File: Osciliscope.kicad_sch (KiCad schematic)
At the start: 65 parts, among them J1 Conn_01x09_Socket, J2 Conn_01x04_Socket, J3 U.FL, J4 Conn_01x04_Socket, J5 USB_C_Receptacle_USB2.0_14P, J6 Conn_01x02_MountingPin, J7 U.FL, SW1 RotaryEncoder_Switch, SW2 SW_SPST, SW3 SW_Nidec_CAS-120A1, SW4 SW_Nidec_CAS-120A1, SW5 RotaryEncoder_Switch, SW6 RotaryEncoder_Switch, U1 MCP1700x-330xxMB, U2 ADC082S101, U3 IP2721, U4 AZ1084-5.0, U5 TLV9061xDBV, U6 TLV9061xDBV, U7 TLV9061xDBV, U8 MCP4251-104E/ML-ND

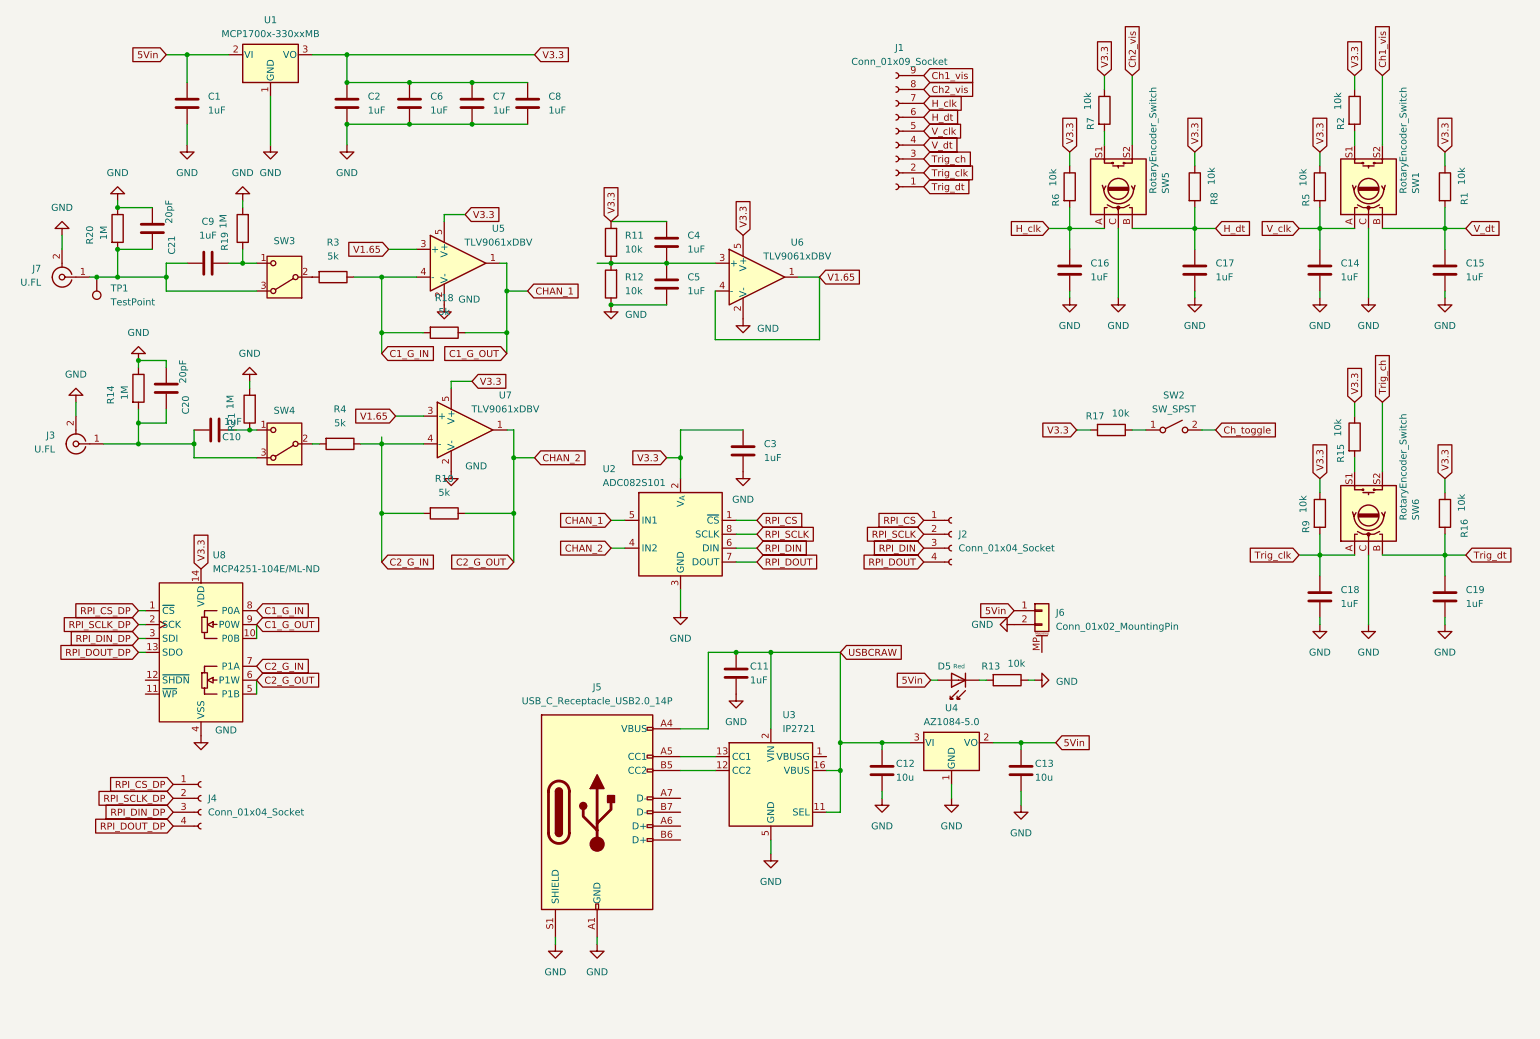
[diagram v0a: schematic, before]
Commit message: more changes to circuit diagram
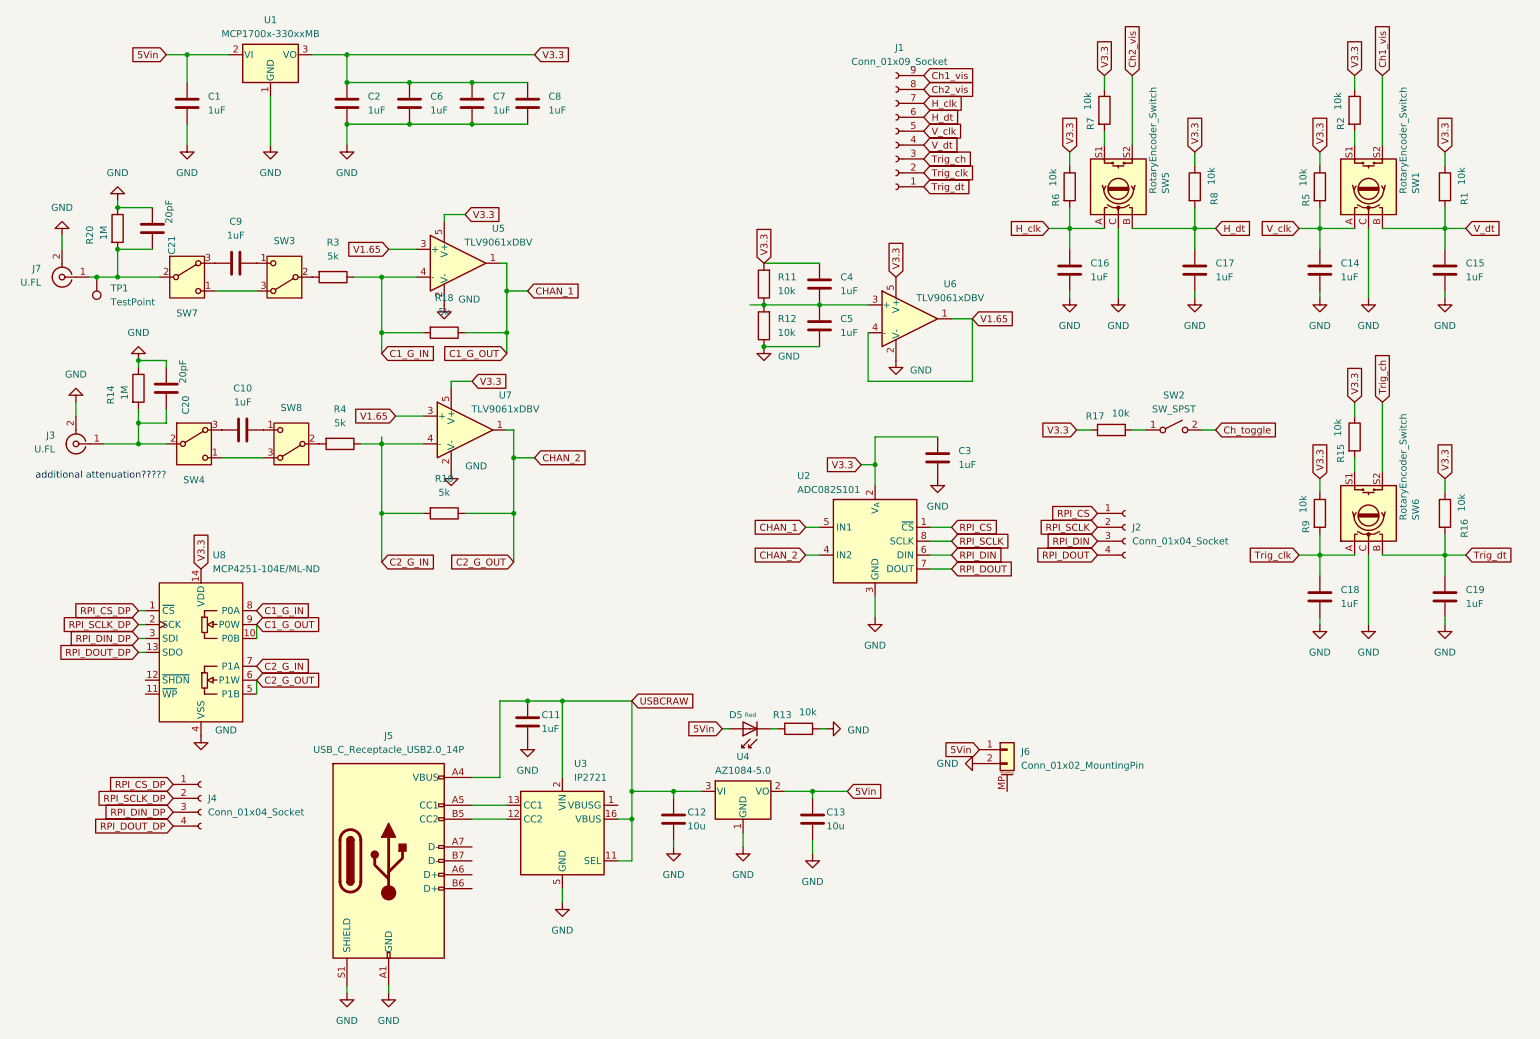
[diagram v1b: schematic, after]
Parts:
- removed R19, R21: 1M, Capacitor_SMD:C_0603_1608Metric, symbol Device:R
- added SW7, SW8: SW_Nidec_CAS-120A1, Button_Switch_SMD:Nidec_Copal_CAS-120A, symbol Switch:SW_Nidec_CAS-120A1
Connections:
- net at C21.2, J7.1 (In), R20.2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: now also SW7.2 (B); no longer C9.1, SW3.3 (A)
- net at C10.2: now also SW8.1 (C); no longer SW4.1 (C)
- net at R4.2: now also SW8.2 (B); no longer SW4.2 (B)
- net at C20.2, J3.1 (In), R14.2: now also SW4.2 (B); no longer C10.1, SW4.3 (A)
- new net: SW4.1 (C), SW8.3 (A)
- new net: SW3.3 (A), SW7.1 (C)
- new net: C9.1, SW7.3 (A)
- new net: C10.1, SW4.3 (A)
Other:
- note added: "additional attenuation?????"
- moved on the sheet: C11, C12, C13, C3, C4, C5, C9, D5, J2, J5, J6, R11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
